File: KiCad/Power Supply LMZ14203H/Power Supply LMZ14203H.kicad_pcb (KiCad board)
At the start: 2 copper layers, 71.8 x 61 mm, 67 parts, among them J1 Power IN, J3 Power OUT, J4 OLED I2C, J5 PDI, J6 OLED, SW1 SW_DIP_x01, U1 INA169, U2 LMZ14203H, U3 L78M12, U4 INA169, U5 UA78M33, U6 ATXMEGA32E5-AU

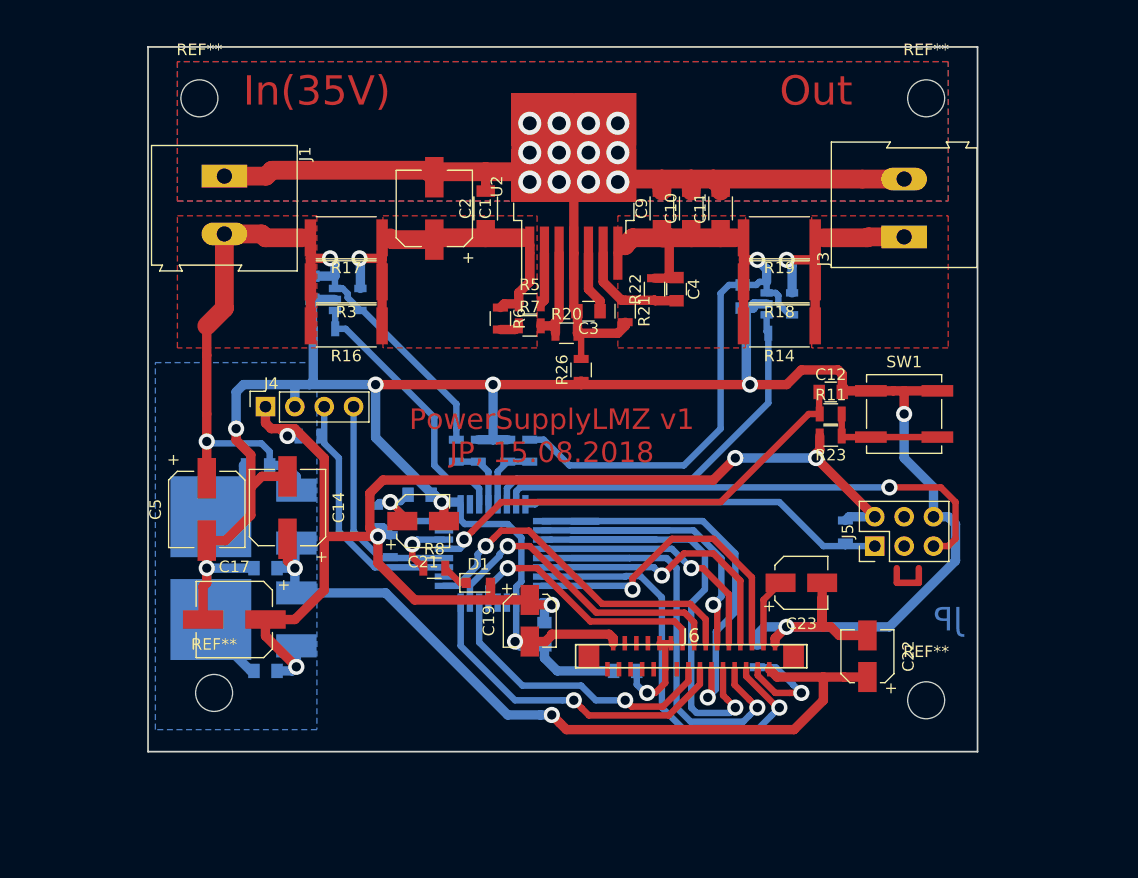
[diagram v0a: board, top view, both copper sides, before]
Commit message: PCB proofing
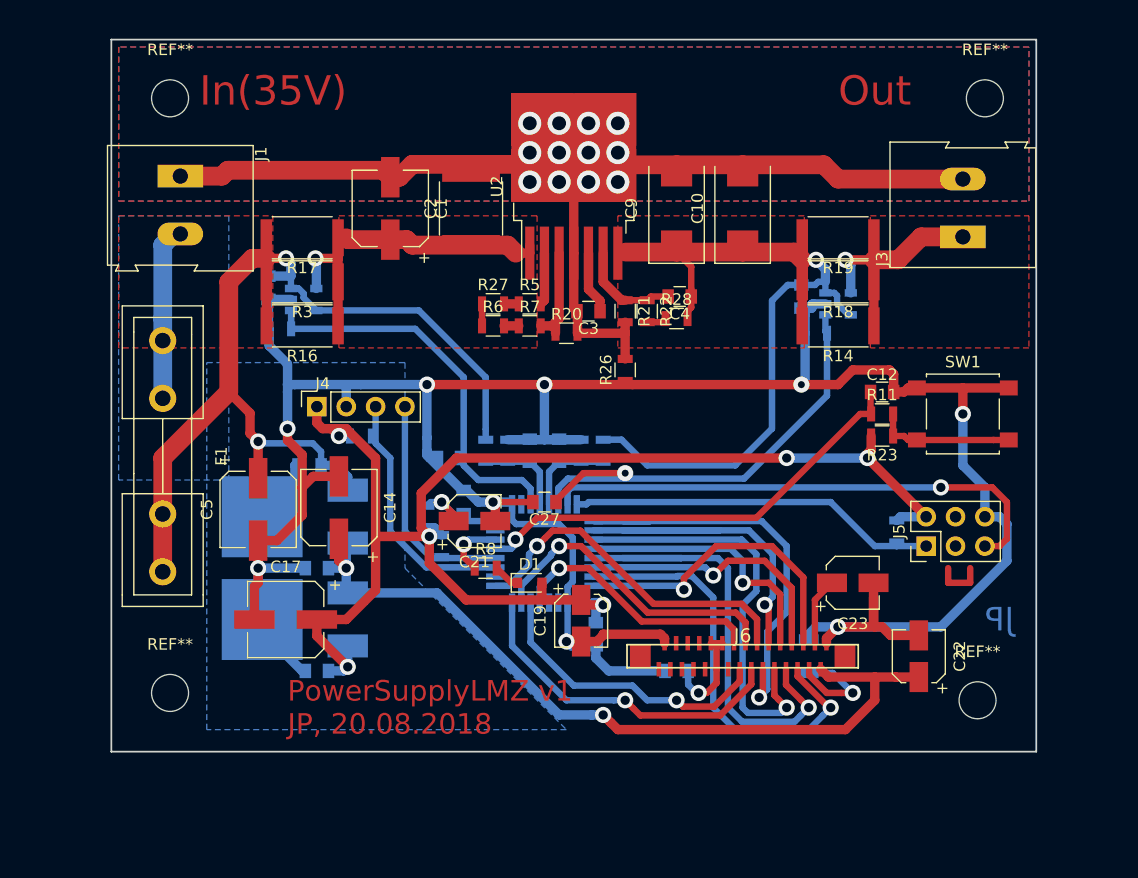
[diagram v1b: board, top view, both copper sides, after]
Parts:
- removed C11: 47u/1-45mESR, Capacitors_SMD:C_1206
- added C15: 100n, Capacitors_SMD:C_0805, B.Cu at (88.3, 84.5)
- added C25: 100n, Capacitors_SMD:C_0805, B.Cu at (81.3, 85.1)
- added C26: 100n, Capacitors_SMD:C_0805, B.Cu at (90.8, 84.5)
- added C27: 100n, Capacitors_SMD:C_0805, F.Cu at (89.5, 88.9)
- added F1: 5A, Fuse_Holders_and_Fuses:Fuseholder5x20_horiz_open_inline_Type-I, F.Cu at (56.5, 74.9)
- added R27: 220k, Resistors_SMD:R_0805, F.Cu at (85.1, 71.8)
- added R28: 15k4, Resistors_SMD:R_0805, F.Cu at (101.0, 73.0)
- C10, C9: footprint Capacitors_SMD:C_1206 -> Capacitors_Tantalum_SMD:CP_Tantalum_Case-D_EIA-7343-31_Reflow
- C2: footprint Capacitors_SMD:C_1206 -> Capacitors_SMD:C_2220
- R21: value 2k43 -> 2k2
- R22: value 34k -> 15k4
- R25: footprint Resistors_SMD:R_0805 -> Resistors_SMD:R_1206
- R5: value 250k -> 30k
- SW1: footprint Buttons_Switches_SMD:SW_SPST_B3SL-1002P -> Buttons_Switches_SMD:SW_SPST_B3S-1000
- moved R12 6.35 mm to (94.6, 84.5)
- moved R13 6.35 mm to (92.7, 84.5)
- moved C8 5.08 mm to (111.8, 71.1)
- moved J3 5.08 mm to (125.7, 66.0)
- moved R14 5.08 mm to (114.9, 73.7)
- moved R15 5.08 mm to (113.0, 74.3)
- moved R18 5.08 mm to (114.9, 69.8)
- moved R19 5.08 mm to (114.9, 66.0)
- moved REF** 5.08 mm to (127.6, 54.0)
- moved SW1 5.08 mm to (125.7, 81.3)
- moved U4 5.08 mm to (114.9, 71.8)
- moved C10 4.45 mm to (106.7, 63.5)
- moved C12 4.45 mm to (118.7, 79.4)
- moved C17 4.45 mm to (67.2, 99.1)
- moved C18 4.45 mm to (94.0, 100.3)
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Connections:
- J1 pad 2: POWER_IN -> Net-(F1-Pad1)
- J5 pad 3: Net-(J5-Pad3) -> (no net)
- J5 pad 4: Net-(J5-Pad4) -> (no net)
- J6 pad 18: Net-(J6-Pad18) -> (no net)
- J6 pad 22: Net-(J6-Pad22) -> (no net)
- J6 pad 23: Net-(J6-Pad23) -> (no net)
- J6 pad 24: Net-(J6-Pad24) -> (no net)
- J6 pad 25: Net-(J6-Pad25) -> (no net)
- J6 pad 26: Net-(J6-Pad26) -> (no net)
- J6 pad 27: Net-(J6-Pad27) -> (no net)
- J6 pad 28: Net-(J6-Pad28) -> (no net)
- J6 pad 30: Net-(J6-Pad30) -> (no net)
- R22 pad 2: Net-(C10-Pad1) -> Net-(R22-Pad2)
- R5 pad 1: Net-(C1-Pad1) -> Net-(R27-Pad2)
- U6 pad 19: Net-(U6-Pad19) -> (no net)
- U6 pad 2: Net-(U6-Pad2) -> (no net)
- U6 pad 20: Net-(U6-Pad20) -> (no net)
- U6 pad 26: Net-(U6-Pad26) -> (no net)
- U6 pad 31: Net-(U6-Pad31) -> (no net)
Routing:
- net POWER_IN: track 72.2 -> 91.1 mm
- net Net-(F1-Pad1): track 0.00 -> 15.3 mm
- net GND: track 247.9 -> 258.7 mm
- net GNDA: track 122.0 -> 132.6 mm
- net IN_Current: track 23.9 -> 34.2 mm
- net OUT_Current: track 34.7 -> 42.6 mm, vias 0 -> 1
- net /OLED_D2: track 43.6 -> 36.3 mm
- net Net-(R11-Pad2): track 10.2 -> 12.2 mm
- net IN_Voltage: track 5.96 -> 7.86 mm
- net OUT_Voltage: track 5.96 -> 7.86 mm
- net Net-(R22-Pad2): track 0.00 -> 1.72 mm
- net Net-(C1-Pad1): track 33.6 -> 32.2 mm
- net Net-(R27-Pad2): track 0.00 -> 1.27 mm
- net /+3.3VA: track 10.6 -> 9.44 mm
- net /OLED_D3: track 22.7 -> 23.8 mm
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- added copper zone on B.Cu, net Net-(F1-Pad1)
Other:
- board size 71.8 x 61 mm -> 80 x 61.6 mm
- board text added: "PowerSupplyLMZ v1 JP, 20.08.2018"
- board text removed: "PowerSupplyLMZ v1 JP, 15.08.2018"

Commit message: PCB proofing
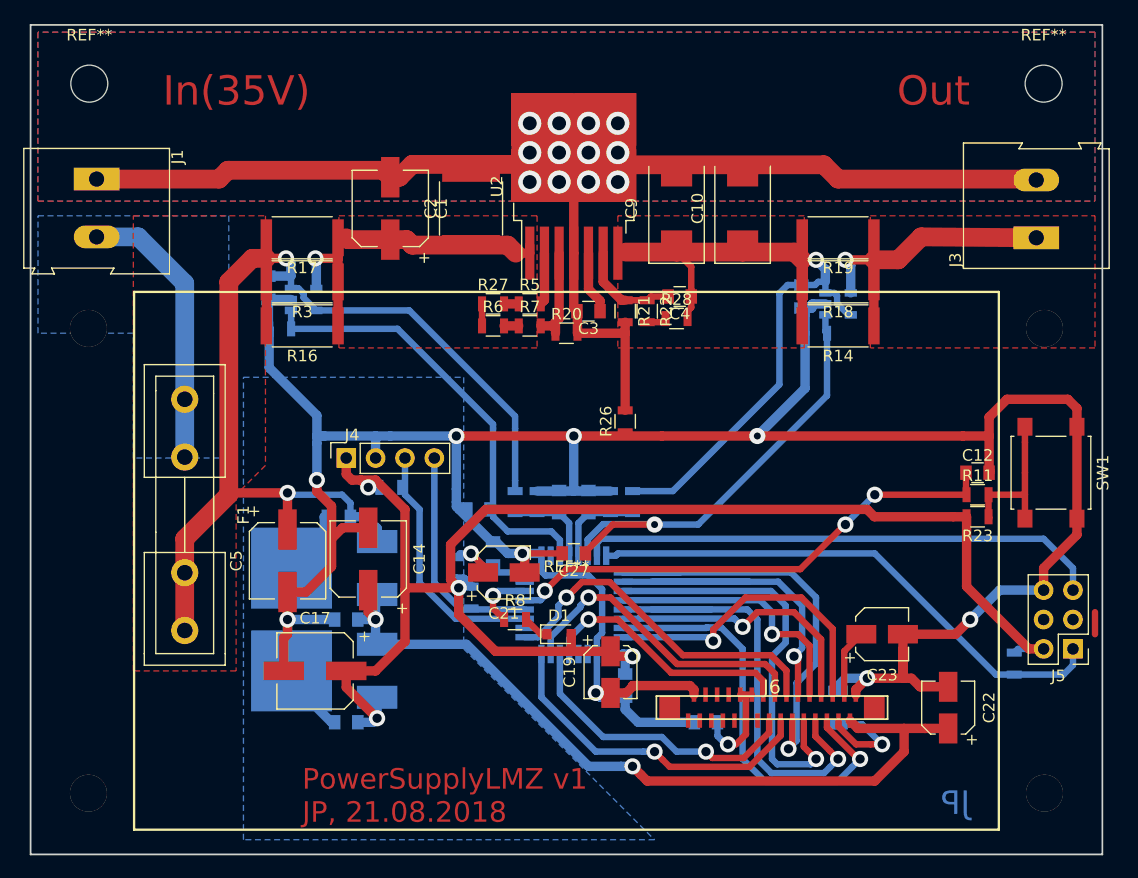
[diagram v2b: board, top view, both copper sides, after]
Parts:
- removed the REF** at (57.1, 105.4)
- removed the REF** at (127.0, 106.0)
- added REF**: RET012864LYPP3N, JPDisplays:RET012864LYPP3N, F.Cu at (91.4, 94.0)
- moved J5 15.5 mm to (135.3, 101.6), turned to 180 degrees
- moved R24 15.3 mm to (130.2, 102.9)
- moved C12 10.8 mm to (127.0, 86.4)
- moved R11 10.8 mm to (127.0, 88.3)
- moved R23 10.8 mm to (127.0, 90.2)
- moved SW1 9.16 mm to (133.3, 86.4), turned to 270 degrees
- moved J1 7.24 mm to (50.8, 61.0)
- moved REF** 7.10 mm to (50.2, 52.7)
- moved J3 6.35 mm to (132.1, 66.0)
- moved F1 5.43 mm to (58.4, 80.0)
- moved REF** 5.24 mm to (132.7, 52.7)
- moved C13 5.12 mm to (72.4, 99.1)
- moved C15 5.12 mm to (90.8, 88.9)
- moved C16 5.12 mm to (72.4, 108.0)
- moved C5 5.12 mm to (67.3, 94.0)
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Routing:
- net GNDA: track 132.6 -> 150.7 mm
- net GND: track 258.7 -> 273.4 mm
- net PDI_CLK: track 32.2 -> 46.5 mm
- net +3V3: track 123.5 -> 135.5 mm, vias 6 -> 4
- net Net-(F1-Pad1): track 15.3 -> 24.3 mm
- net POWER_IN: track 91.1 -> 99.9 mm
- net POWER_OUT: track 21.7 -> 28.0 mm
- net SWITCH: track 39.5 -> 44.3 mm, vias 1 -> 3
- net IN_Current: track 34.2 -> 38.8 mm
- net Net-(C10-Pad1): track 70.6 -> 66.2 mm
- net (no net): track 4.45 -> 1.91 mm
- net OUT_Current: track 42.6 -> 41.5 mm
- net Net-(R11-Pad2): track 12.2 -> 13.1 mm
- net PDI_DATA: track 45.1 -> 45.4 mm, vias 1 -> 0
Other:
- board size 80 x 61.6 mm -> 92.7 x 71.8 mm
- board text added: "PowerSupplyLMZ v1 JP, 21.08.2018"
- board text removed: "PowerSupplyLMZ v1 JP, 20.08.2018"
